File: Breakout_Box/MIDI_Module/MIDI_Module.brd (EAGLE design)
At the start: 55 x 80 mm, 71 parts, among them T1 2N2222, T2 2N2222, U1 LMV324, U2 LMV324, U3 MIC5205-5.0YM5-TR, U4 MIC5205-3.3YM5-TR

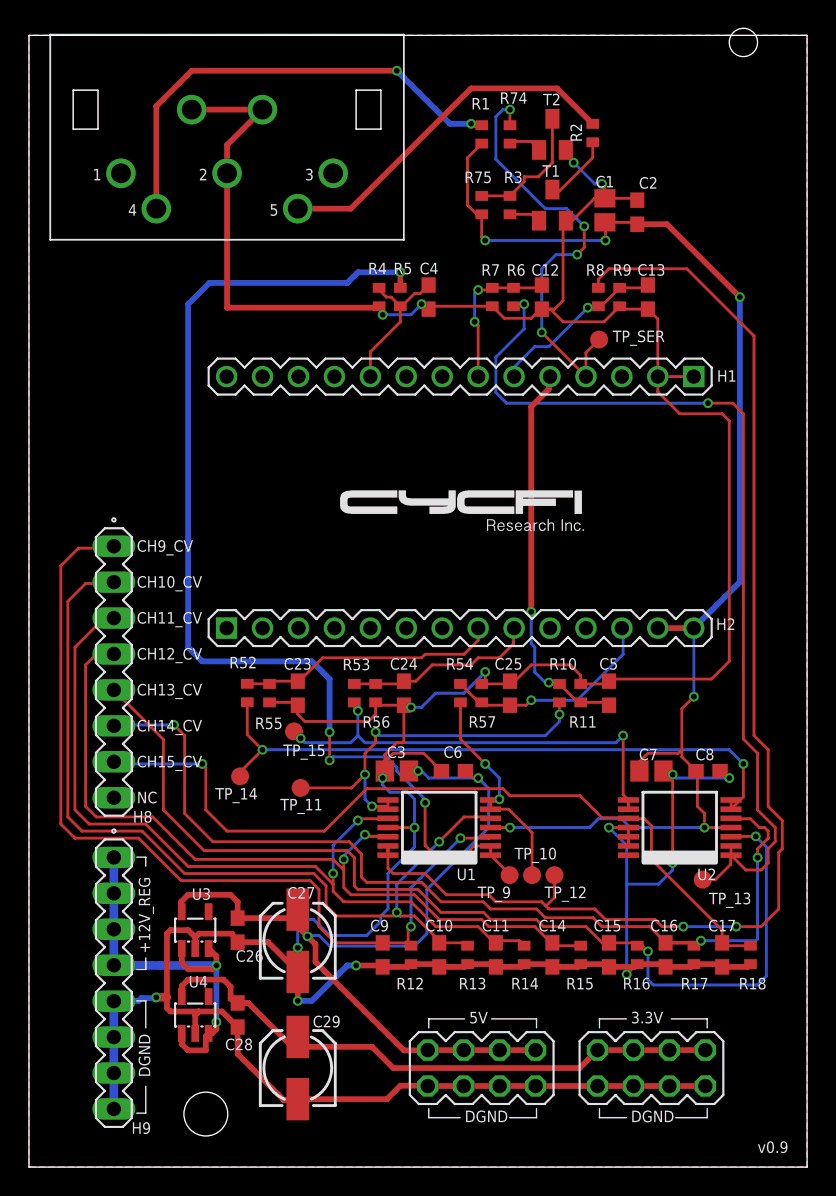
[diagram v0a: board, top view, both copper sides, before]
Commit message: Licenses
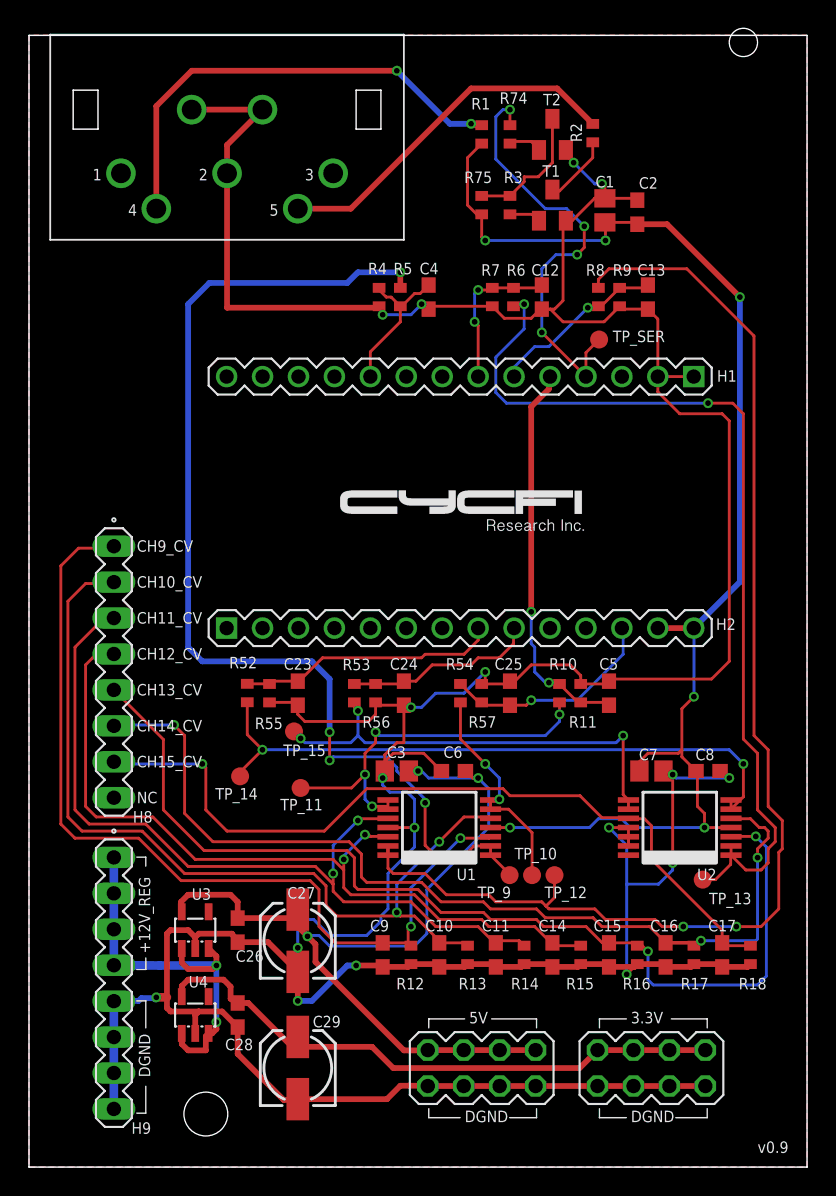
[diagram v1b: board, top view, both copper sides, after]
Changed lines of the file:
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@@
 <board>
 <plain>
-<wire x1="0" y1="0" x2="55" y2="0" width="0" layer="20"/>
-<wire x1="55" y1="0" x2="55" y2="80" width="0" layer="20"/>
-<wire x1="55" y1="80" x2="0" y2="80" width="0" layer="20"/>
-<wire x1="0" y1="80" x2="0" y2="0" width="0" layer="20"/>
+<wire x1="0" y1="0" x2="55" y2="0" width="0.1" layer="20"/>
+<wire x1="55" y1="0" x2="55" y2="80" width="0.1" layer="20"/>
+<wire x1="55" y1="80" x2="0" y2="80" width="0.1" layer="20"/>
+<wire x1="0" y1="80" x2="0" y2="0" width="0.1" layer="20"/>
 <text x="7.62" y="43.4975" size="0.8128" layer="25" ratio="13">CH9_CV</text>
 <text x="7.62" y="40.9575" size="0.8128" layer="25" ratio="13">CH10_CV</text>
